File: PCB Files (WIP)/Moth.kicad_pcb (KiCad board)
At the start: 2 copper layers, 220.6 x 118.4 mm, 58 parts, among them J1 Conn_01x02, J2 JTAG_TC2030, J3 DuPont Connector, J4 Left Ribbon, J5 Right Ribbon, SW1 Boot, U1 XC6206, U2 X05A26H12G, U3 RP2040, U4 W25Q128JVS, Y1 12MHz

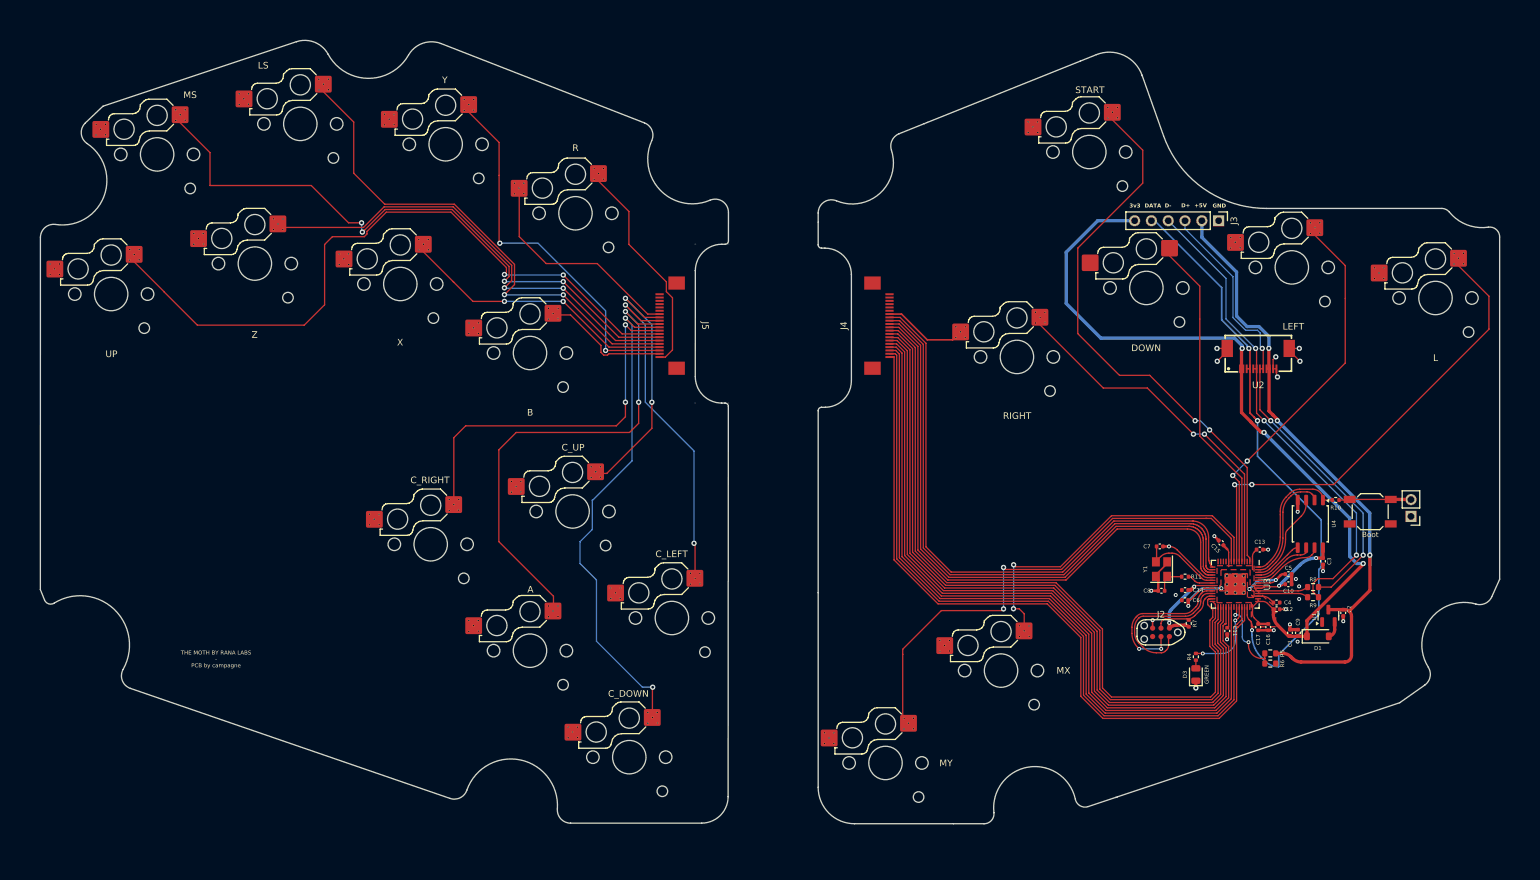
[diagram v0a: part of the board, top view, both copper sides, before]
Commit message: PCB files possibly done pending testing
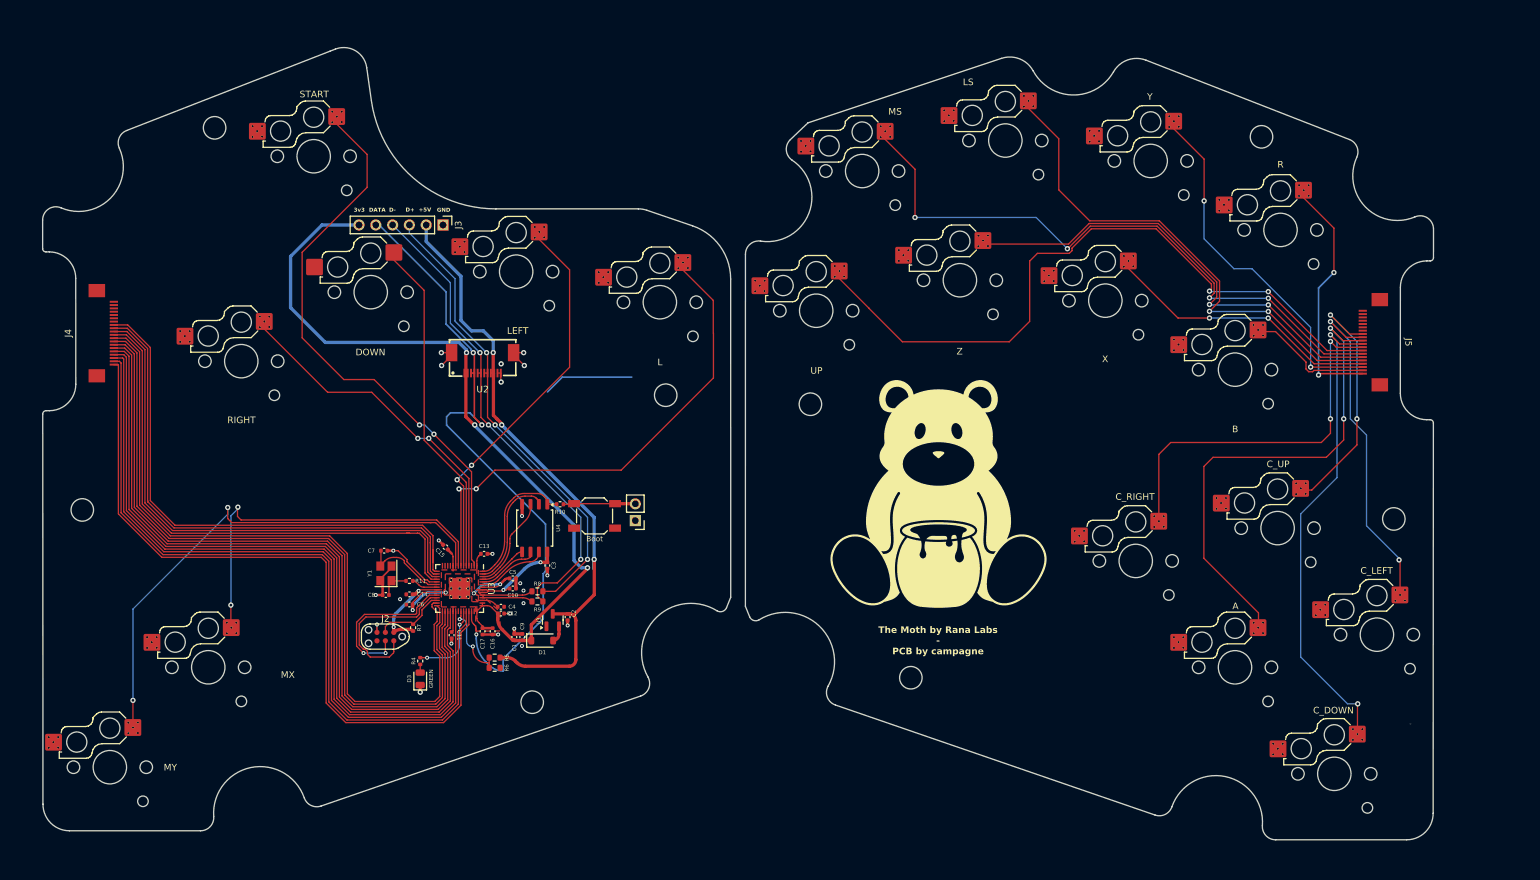
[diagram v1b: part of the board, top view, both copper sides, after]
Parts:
- moved MX1 119.8 mm to (65.2, 129.8)
- moved J4 117.2 mm to (46.1, 79.3)
- moved C10 117.2 mm to (111.3, 117.8)
- moved C12 117.2 mm to (109.5, 121.6)
- moved C13 117.2 mm to (106.9, 112.6)
- moved C2 117.2 mm to (119.6, 122.2)
- moved C3 117.2 mm to (116.5, 114.4)
- moved C4 117.2 mm to (109.5, 120.6)
- moved C5 117.2 mm to (111.3, 116.3)
- moved C7 117.2 mm to (91.8, 112.1)
- moved C8 117.2 mm to (92.1, 118.8)
- moved C9 117.2 mm to (112.7, 125.2)
- moved J1 117.2 mm to (129.8, 107.6)
- moved L1 117.2 mm to (133.5, 74.6)
- moved R5 117.2 mm to (108.5, 128.3)
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- renumbered A to A1, B to B1, C_DOWN to C_DOWN1, C_LEFT to C_LEFT1, C_RIGHT to C_RIGHT1, C_UP to C_UP1, DOWN to DOWN1, L to L1, LEFT to LEFT1, LS to LS1, MS to MS1, MX to MX1, MY to MY1, R to R1, RIGHT to RIGHT1, START to START1, UP to UP1, X to X1, Y to Y2, Z to Z1
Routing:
- net GND: track 103.2 -> 76.0 mm
- net A RIBBON: track 91.5 -> 80.8 mm
- net C_LT RIBBON: track 91.6 -> 81.0 mm
- net C_DN RIBBON: track 91.3 -> 81.5 mm
- net DATA: track 92.7 -> 102.5 mm
- net C_UP RIBBON: track 91.5 -> 82.8 mm
- net M1: track 52.8 -> 58.8 mm
- net L: track 72.7 -> 76.6 mm
- net R: track 33.8 -> 37.7 mm, vias 0 -> 2
- net MS RIBBON: track 110.2 -> 113.0 mm
- net M2: track 78.3 -> 81.1 mm
- net C_RT RIBBON: track 111.3 -> 113.9 mm
- net UP RIBBON: track 110.8 -> 113.4 mm
- net Z RIBBON: track 111.0 -> 113.6 mm
- net LS RIBBON: track 111.7 -> 114.2 mm
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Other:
- board size 220.6 x 118.4 mm -> 210.2 x 119.7 mm
- board text added: "The Moth by Rana Labs - PCB by campagne"
- board text removed: "THE MOTH BY RANA LABS - PCB by campagne"
